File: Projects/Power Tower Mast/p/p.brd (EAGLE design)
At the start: 16.5 x 21.6 mm, 32 parts

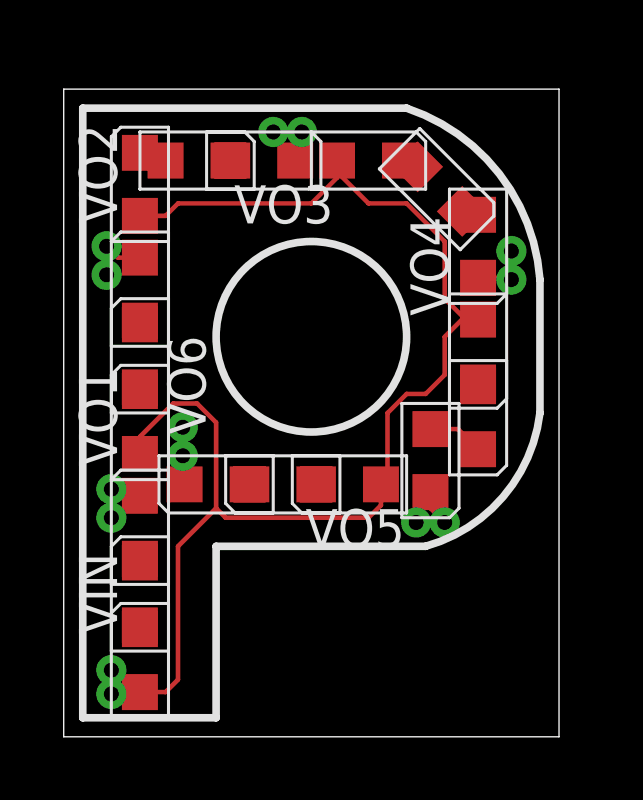
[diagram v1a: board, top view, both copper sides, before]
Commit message: final updates before fab.  added new letters for future projects.
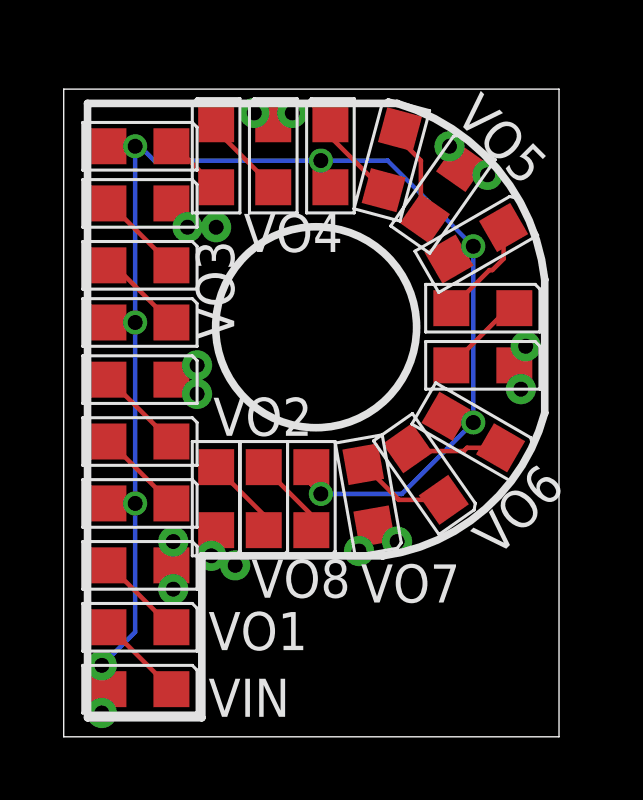
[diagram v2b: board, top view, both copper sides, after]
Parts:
- added LED19, LED20, LED21, LED22, LED23, LED24: (no value), CyberRailGuru:LED_0805
- added VO13, VO14, VO15, VO16: (no value), CyberRailGuru:P1-20
- moved VO9 14.3 mm to (3.65, 6.51)
- moved VO11 11.9 mm to (5.08, 17.0)
- moved VO5 11.7 mm to (14.1, 18.7)
- moved VO6 11.5 mm to (15.2, 11.6)
- moved VO8 11.5 mm to (5.71, 5.71)
- moved VO10 11.1 mm to (4.45, 12.4)
- moved VO12 11.1 mm to (7.62, 20.8)
- moved VO4 10.2 mm to (6.35, 20.8)
- moved LED18 9.74 mm to (14.0, 12.4), turned to 270 degrees
- moved VO7 9.68 mm to (11.1, 6.51)
- moved LED16 9.08 mm to (13.8, 16.5), turned to 300 degrees
- moved LED14 9.07 mm to (10.9, 19.2), turned to 345 degrees
- moved LED15 8.94 mm to (12.6, 18.1), turned to 325 degrees
- moved LED17 8.89 mm to (14.0, 14.3), turned to 270 degrees
- moved LED13 8.16 mm to (8.89, 19.4), turned to 0 degrees
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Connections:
- new net N$11: LED24.C, VO16.TP, VO8.TP
- new net N$12: LED21.C, VO15.TP, VO7.TP
- new net N$3: LED19.C, LED20.A
- new net N$4: LED20.C, LED21.A
- new net N$7: LED22.C, LED23.A
- new net N$8: LED23.C, LED24.A
- net VIN: now also LED19.A, LED22.A
- net VOUT1: now also VO9.TP; no longer VO7.TP
- net VOUT2: now also VO10.TP; no longer VO8.TP
- net VOUT3: now also VO11.TP; no longer VO9.TP
- net VOUT4: now also VO12.TP; no longer VO10.TP
- net VOUT5: now also VO13.TP; no longer VO11.TP
- net VOUT6: now also VO14.TP; no longer VO12.TP
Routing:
- net VIN: track 46.2 -> 51.8 mm, vias 0 -> 7
- net N$22: track 0.12 -> 3.47 mm
- net N$3: track 0.00 -> 3.18 mm
- net N$4: track 0.00 -> 3.18 mm
- net N$9: track 0.12 -> 2.95 mm
- net N$1: track 0.12 -> 2.95 mm
- net N$2: track 0.12 -> 2.95 mm
- net N$6: track 0.12 -> 2.95 mm
- net N$5: track 0.12 -> 2.95 mm
- net N$18: track 0.12 -> 2.93 mm
- net N$21: track 0.12 -> 2.89 mm
- net N$8: track 0.00 -> 2.76 mm
- net N$7: track 0.00 -> 2.76 mm
- net N$13: track 0.57 -> 2.89 mm
- net N$12: track 0.00 -> 2.01 mm
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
